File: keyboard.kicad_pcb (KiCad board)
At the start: 2 copper layers, 108.2 x 96.2 mm, 68 parts, among them J2 TYPE-C-31-M-12, U1 ATmega32U4-A, Y1 Crystal_GND24_Small

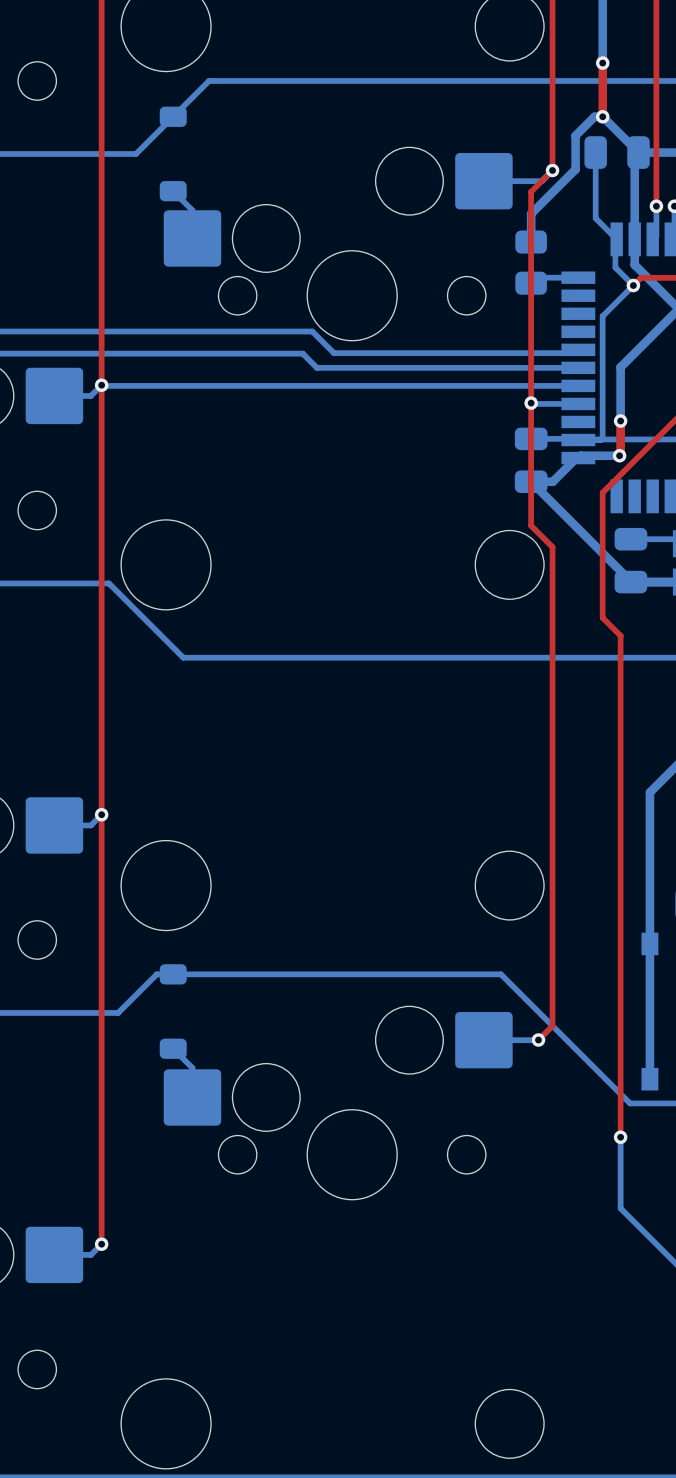
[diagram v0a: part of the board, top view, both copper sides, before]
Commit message: fixFlip
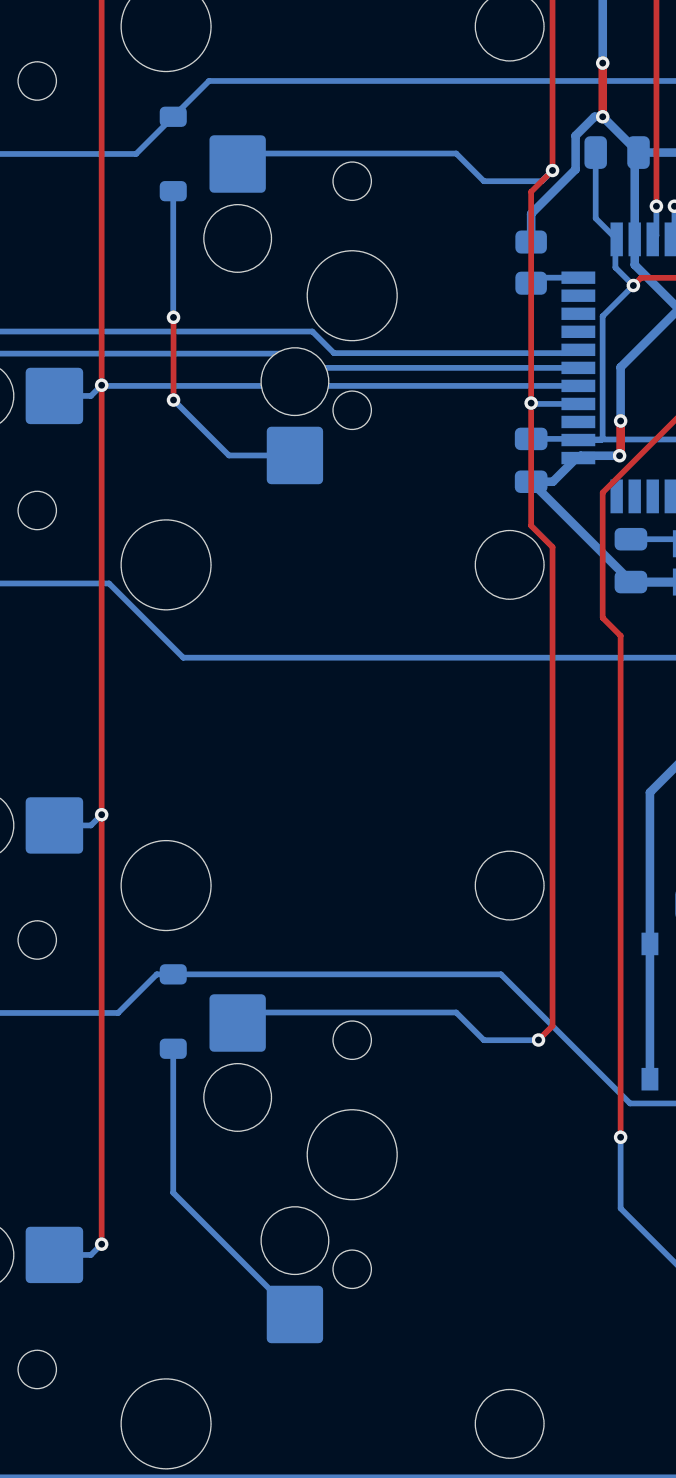
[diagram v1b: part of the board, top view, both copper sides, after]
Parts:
- Key_+1, Key_enter1: footprint Button_Switch_Keyboard:MX-Hotswap-2U-Vertical-ReversedStabilizers -> Button_Switch_Keyboard:MX-Hotswap-2U-ReversedStabilizers
- turned Key_+1 to -90 degrees
- turned Key_enter1 to -90 degrees
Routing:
- net Y3: track 79.1 -> 102.4 mm
- net Net-(D12-A): track 2.45 -> 15.7 mm, vias 0 -> 2
- net Net-(D16-A): track 2.51 -> 14.0 mm
